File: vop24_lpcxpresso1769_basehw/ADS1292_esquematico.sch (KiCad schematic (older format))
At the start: 45 parts

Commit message: Primera versión esquematico sin revisar
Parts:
- removed J? (x3): Conn_01x02, symbol Connector_Generic:Conn_01x02
- added J5, J6, J7: Conn_01x04, symbol Connector_Generic:Conn_01x04
- added R11, R12, R13: 33k, symbol Device:R_Small
- added U5, U6, U7: LM334, symbol vop24_lpcxpresso1769_basehw-rescue:LM334
- gave numbers to parts that had none: 42
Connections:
- net labels removed: GNDD
- wire segments 165 -> 198
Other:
- moved on the sheet: C12, C13, C14, C15, C16, C17, C18, C19, C20, R14, R15, R16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

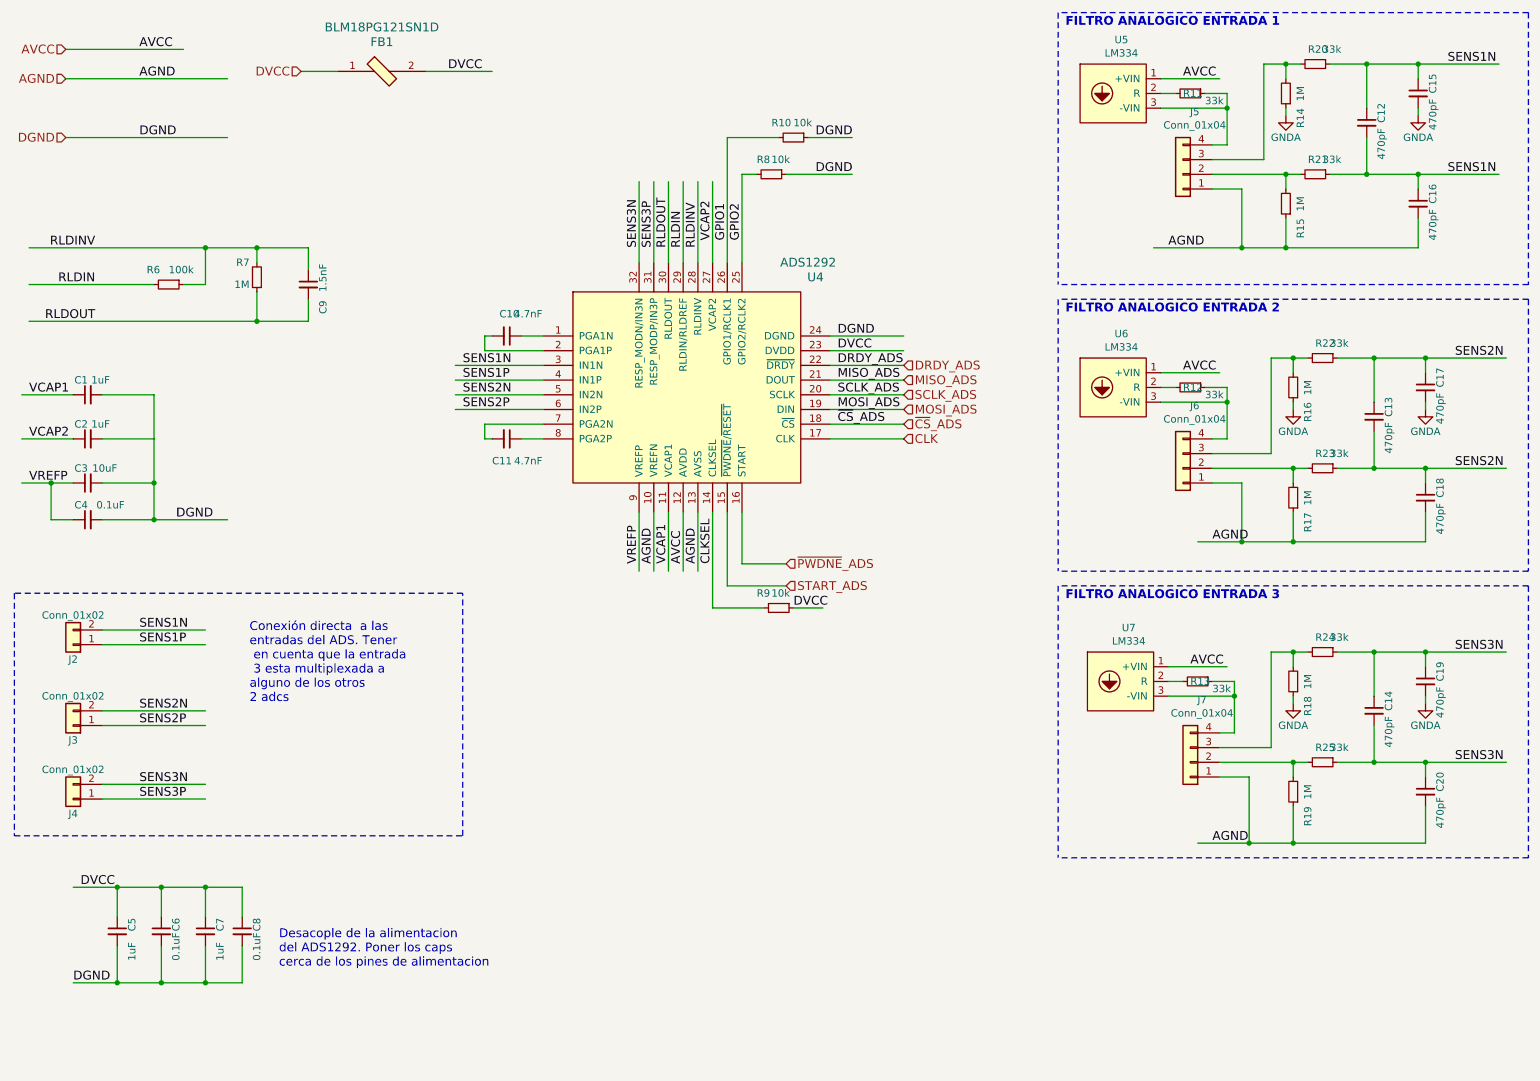
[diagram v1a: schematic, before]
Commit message: Algunas correcciones sobre el esquemático. Falta terminar de revisar algunos conflictos del DRC
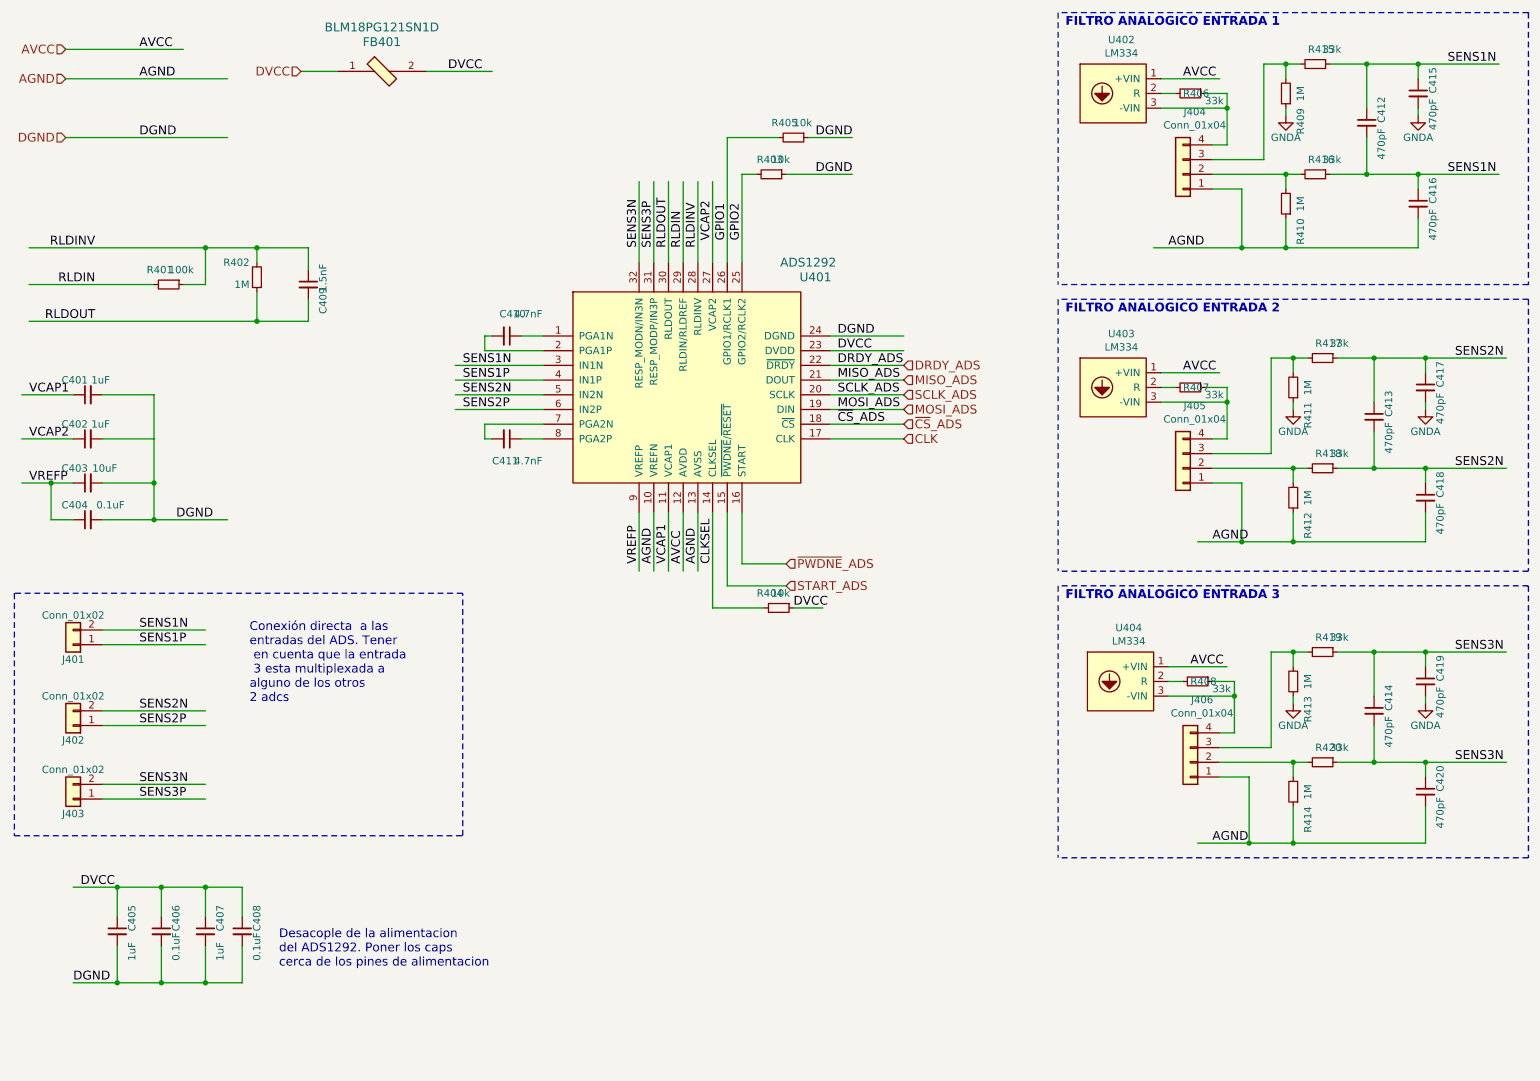
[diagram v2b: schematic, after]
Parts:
- renumbered C1 to C401, C2 to C402, C3 to C403, C4 to C404, C5 to C405, C6 to C406, C7 to C407, C8 to C408, C9 to C409, C10 to C410, C11 to C411, C12 to C412, C13 to C413, C14 to C414, C15 to C415, C16 to C416, C17 to C417, C18 to C418, C19 to C419, C20 to C420, FB1 to FB401, J2 to J401, J3 to J402, J4 to J403, J5 to J404, J6 to J405, J7 to J406, R6 to R401, R7 to R402, R8 to R403, R9 to R404, R10 to R405, R11 to R406, R12 to R407, R13 to R408, R14 to R409, R15 to R410, R16 to R411, R17 to R412, R18 to R413, R19 to R414, R20 to R415, R21 to R416, R22 to R417, R23 to R418, R24 to R419, R25 to R420, U4 to U401, U5 to U402, U6 to U403, U7 to U404
